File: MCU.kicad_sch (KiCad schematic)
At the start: 44 parts, among them J4 SWD, J5 SSD1306, SW1 EC11E15244G1, U12 FT234XD, U2 STM32G474CEUx, Y1 8M

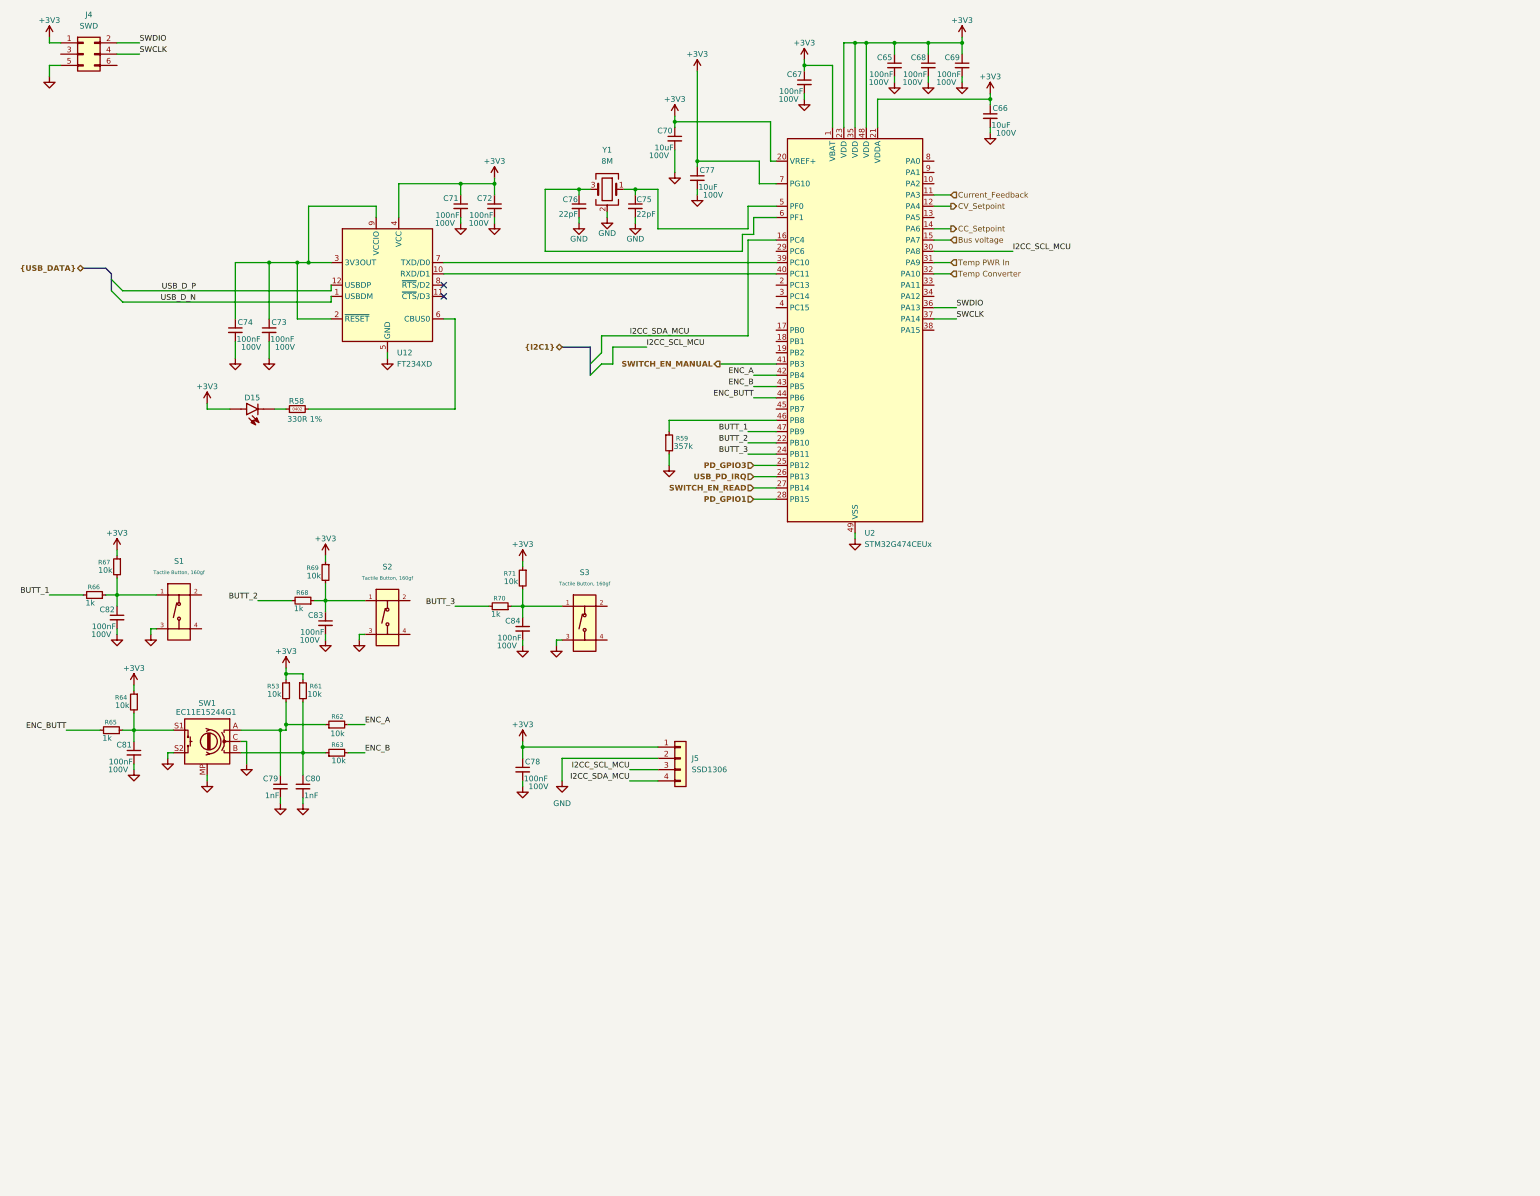
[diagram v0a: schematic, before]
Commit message: Started routing
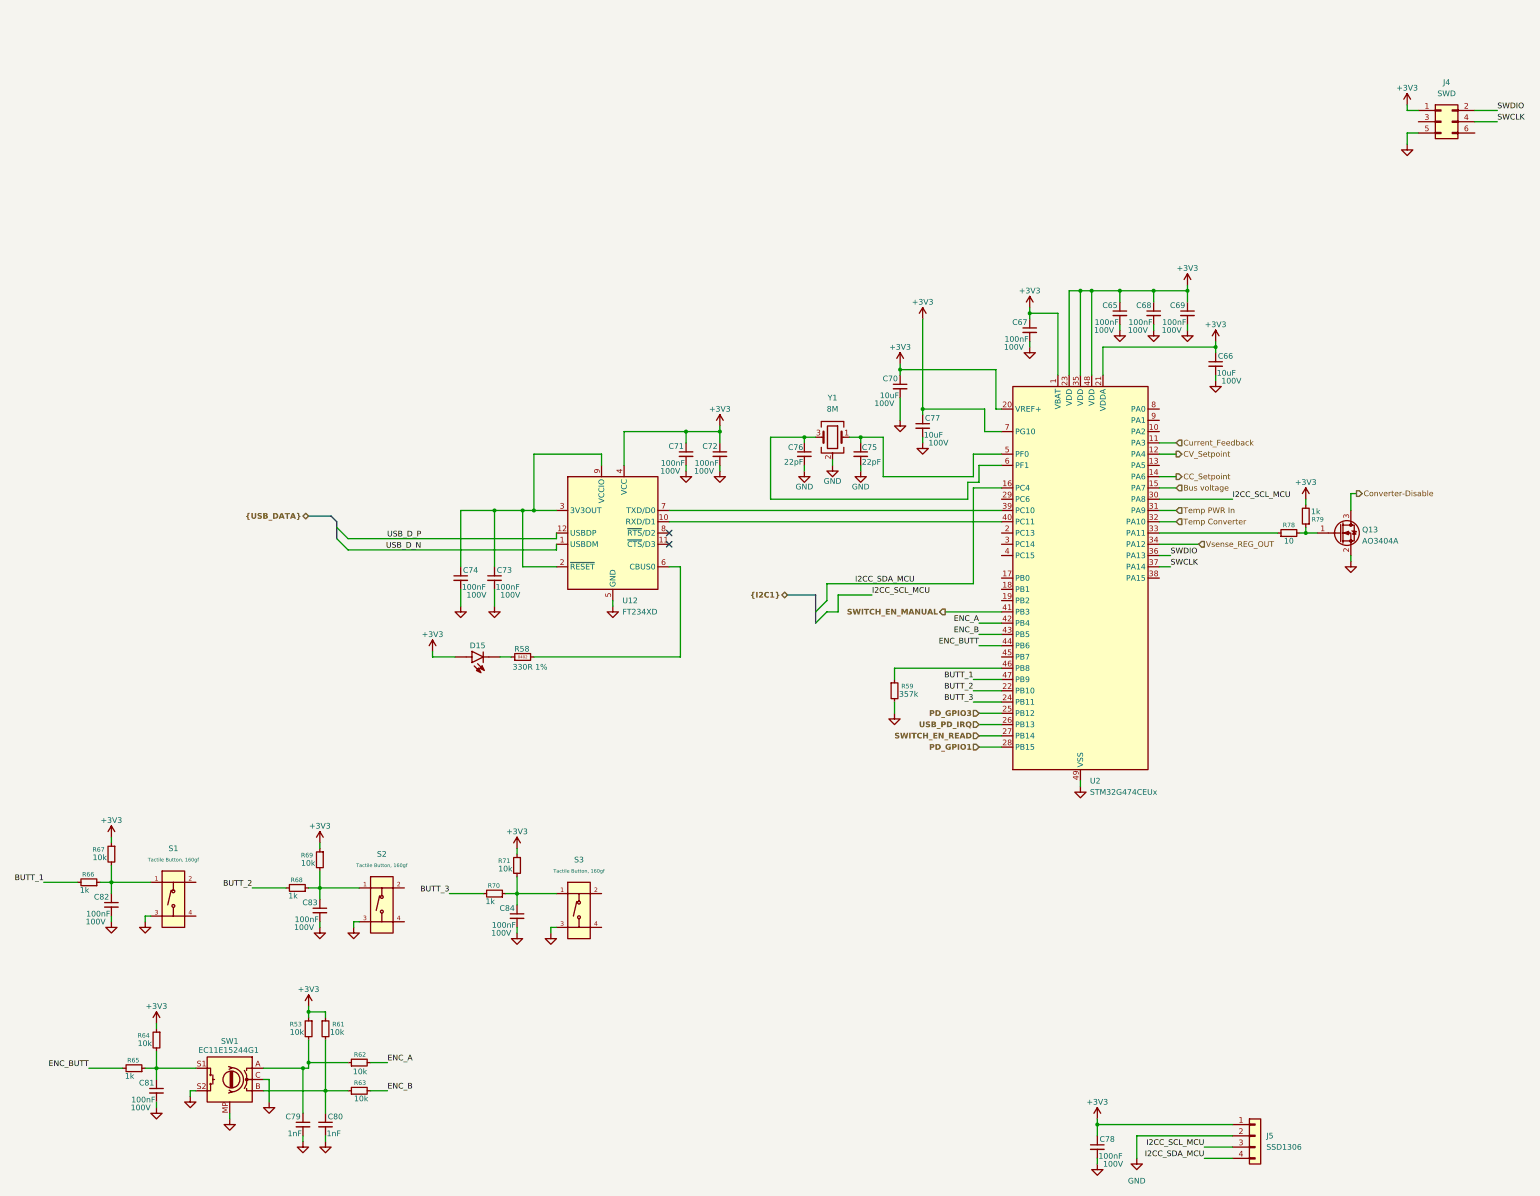
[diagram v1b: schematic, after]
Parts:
- added Q13: AO3404A, Altium_port:sot-23-3L_103p_300x130x110_n, symbol Transistor_FET_Other:Q_NMOS_Depletion_GSD
- added R78: 10, Resistor_SMD:R_0402_1005Metric, symbol Device:R_Small
- added R79: 1k, Resistor_SMD:R_0402_1005Metric, symbol Device:R_Small
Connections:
- net +3V3: now also R79.2
- net GND: now also Q13.2 (S)
- net at U2.33 (PA11): now also R78.1
- net Vsense_REG_OUT: now reaches U2.34 (PA12)
- new net: Q13.1 (G), R78.2, R79.1
- new net Converter-Disable: Q13.3 (D)
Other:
- title: (none) -> Nitride-Nano
- moved on the sheet: C65, C66, C67, C68, C69, C70, C71, C72, C73, C74, C75, C76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
